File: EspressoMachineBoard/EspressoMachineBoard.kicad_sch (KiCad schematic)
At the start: 70 parts, among them J1 USB_C_Receptacle_USB2.0_14P, J2 Conn_01x04_Pin, J3 Conn_01x02_Pin, J4 Conn_01x02_Pin, J5 Conn_01x08_Pin, J6 Conn_01x14_Pin, J7 Conn_01x14_Pin, Q1 NMOS, Q2 NMOS, Q7 NMOS, Q8 NMOS, Q9 NMOS, SW1 SW_Push, SW2 SW_Push, SW3 PEC11R-4215K-S0012, SW4 SW_SPDT, U1 ESP32-S3-WROOM-2, U2 AP7361C-33E, U3 LM358_DFN, U5 74AHC1G08GW,125, U6 LM4040A25IDCKR, U9 LM358_DFN

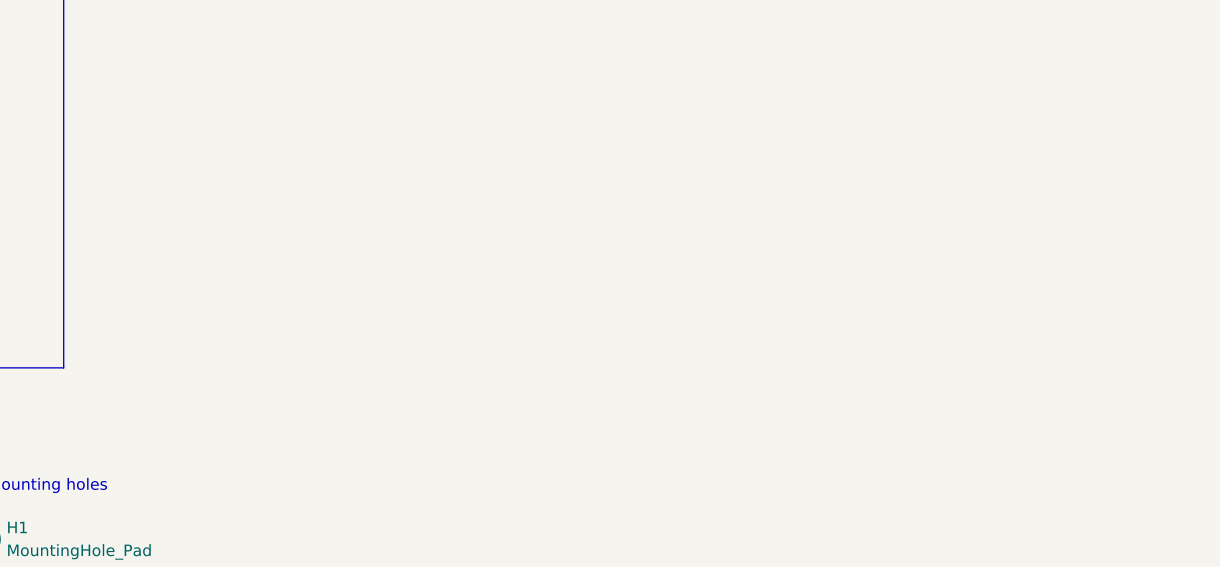
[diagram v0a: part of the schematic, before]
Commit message: Added issues
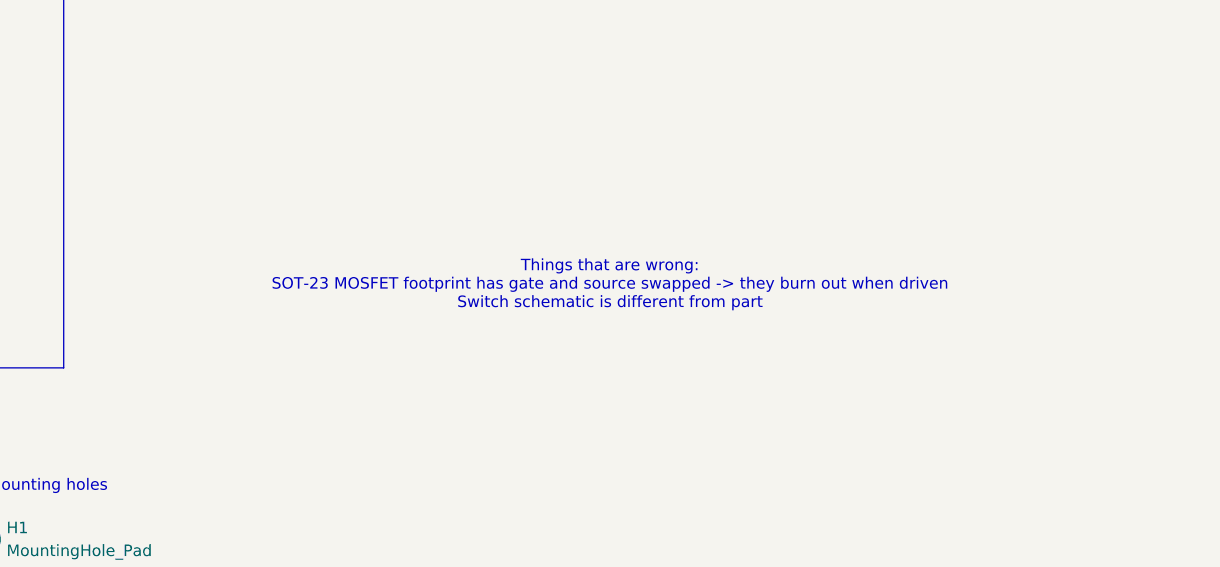
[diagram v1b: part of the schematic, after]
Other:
- note added: "Things that are wrong: SOT-23 MOSFET footprint has gate and source swapped -> they burn out when driven Switch schematic is different from part"
